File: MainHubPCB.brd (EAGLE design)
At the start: 100 x 80.3 mm, 77 parts, among them Q1 600mA/40V, Q2 600mA/40V, Q3 600mA/40V, U1 HX711, U2 HX711, U4 STM32F0XXC1T, U5 PCF8574T/3,512SOT162-1-M, U6 HX711

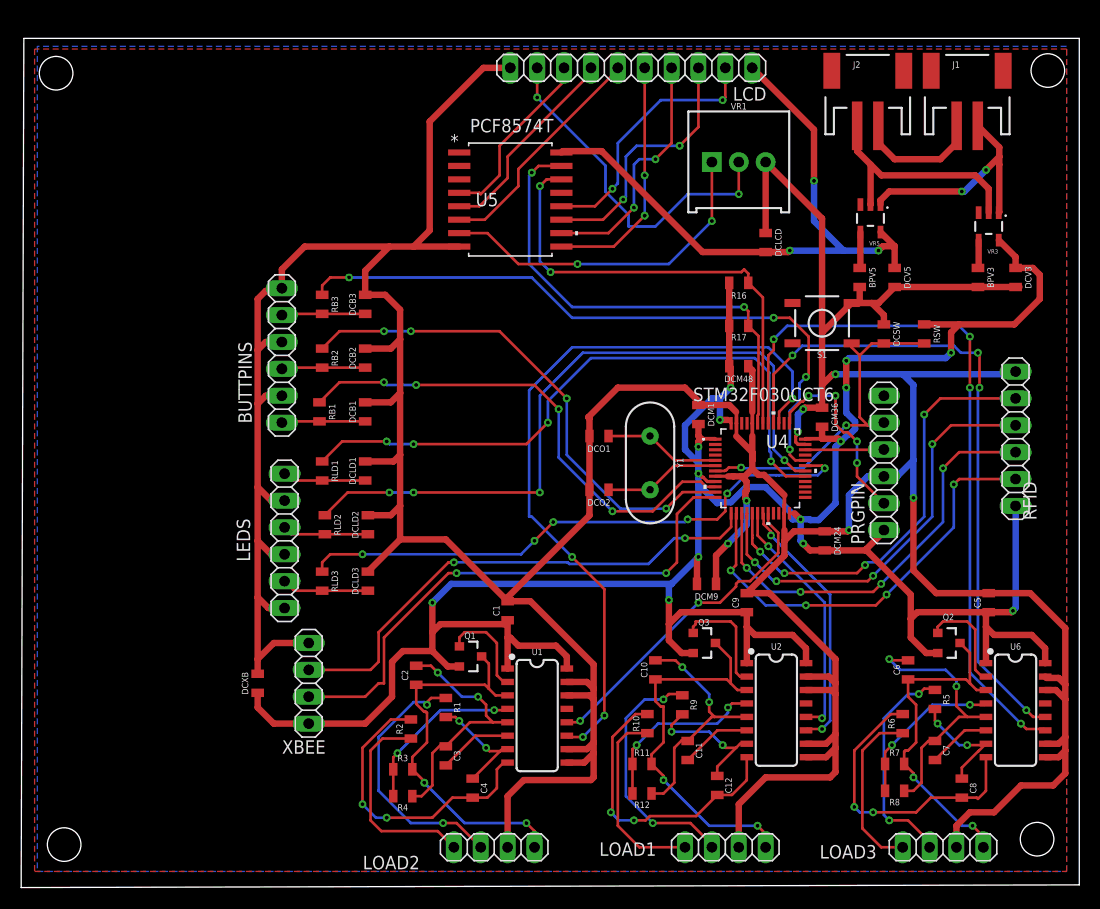
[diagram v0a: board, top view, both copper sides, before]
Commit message: final stuff
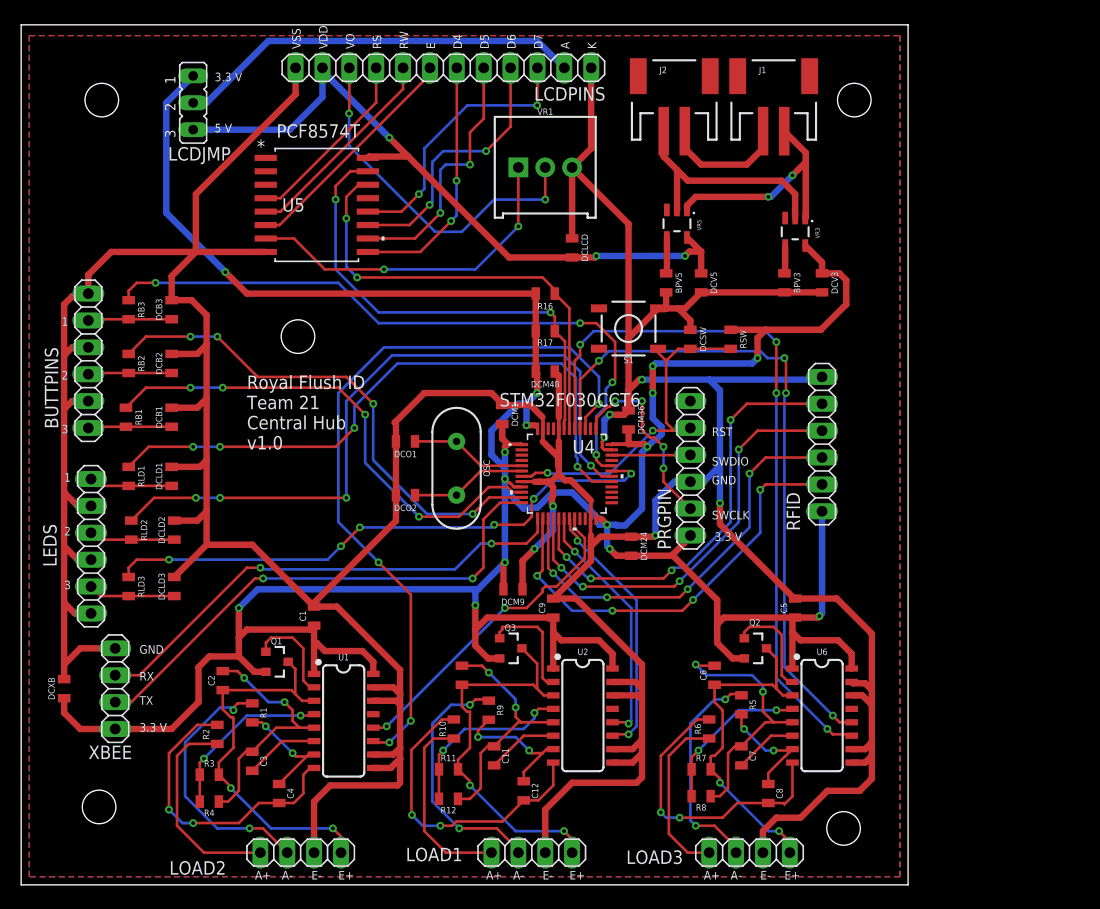
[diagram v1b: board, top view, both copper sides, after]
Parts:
- removed LCD: (no value), pinhead:1X10
- removed Y1: (no value), SparkFun-Clocks:HC49US
- added LCDJMP: (no value), jumper:JP2
- added LCDPINS: (no value), pinhead:1X12
- added OSC: (no value), SparkFun-Clocks:HC49US
- moved DCM1 18.5 mm to (45.5, 44.5)
- moved R16 18.3 mm to (49.5, 55.9)
- moved BPV3 18.3 mm to (72.1, 56.9)
- moved C8 18.3 mm to (70.6, 8.64)
- moved DCV3 18.3 mm to (75.7, 56.9)
- moved RFID 18.3 mm to (75.7, 41.7)
- moved U6 18.3 mm to (75.7, 16.0)
- moved BPV5 18.3 mm to (61.0, 56.9)
- moved BUTTPINS 18.3 mm to (6.35, 49.5)
- moved C10 18.3 mm to (41.7, 19.8)
- moved C12 18.3 mm to (47.5, 8.89)
- moved DCLCD 18.3 mm to (52.1, 60.2)
- moved DCSW 18.3 mm to (63.2, 51.6)
- moved J2 18.3 mm to (61.7, 74.9)
- moved LOAD1 18.3 mm to (48.3, 3.05)
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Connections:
- net A2 renamed TX
- net A3 renamed RX
- net B6 renamed SCL
- net B7 renamed SDA
- net N$12 renamed 3_A-
- net N$13 renamed 3_A+
- net N$17 renamed 3_VDD
- net N$2 renamed 2_A-
- net N$23 renamed 1_A-
- net N$24 renamed 1_A+
- net N$28 renamed 1_VDD
- net N$3 renamed 2_A+
- net N$7 renamed 2_VDD
- removed net B: LCD.9, VR1.2
- removed net D0: LCD.8, U5.4
- removed net D1: LCD.7, U5.5
- removed net D2: LCD.6, U5.6
- new net E: LCDPINS.7, U5.6
- new net POT_A: U5.7, VR1.1
- new net POT_B: LCDPINS.10, VR1.2
- new net RS: LCDPINS.9, U5.4
- new net RW: LCDPINS.8, U5.5
- net A: now also LCDJMP.2, LCDPINS.2; no longer U5.7, VR1.1
- net D4: now also LCDPINS.6; no longer LCD.5
- net D5: now also LCDPINS.5; no longer LCD.4
- net D6: now also LCDPINS.4; no longer LCD.3
- net D7: now also LCDPINS.3; no longer LCD.2
- net GND: now also LCDPINS.1, LCDPINS.12; no longer LCD.10
- net N$21: now also OSC.1; no longer Y1.1
- net N$22: now also OSC.2; no longer Y1.2
- net P3V: now also LCDJMP.1
- net P5V: now also LCDJMP.3, LCDPINS.11; no longer LCD.1
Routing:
- net P3V: track 275.7 -> 328.2 mm, vias 14 -> 15
- net POT_B: track 0.00 -> 33.6 mm, vias 0 -> 2
- net B: track 33.3 -> 0.00 mm, vias 2 -> 0
- net POT_A: track 0.00 -> 32.3 mm, vias 0 -> 2
- net E: track 0.00 -> 22.1 mm
- net D2: track 22.0 -> 0.00 mm
- net RW: track 0.00 -> 19.8 mm
- net D1: track 19.4 -> 0.00 mm
- net RS: track 0.00 -> 17.5 mm
- net D0: track 17.3 -> 0.00 mm
- net P5V: track 60.5 -> 67.7 mm
- net A: track 32.3 -> 38.5 mm, vias 2 -> 0
- net GND: track 510.6 -> 515.8 mm
- net TX: track 51.4 -> 48.9 mm
- net RX: track 48.6 -> 46.9 mm
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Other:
- board size 100 x 80.3 mm -> 83.8 x 81.3 mm
- board text added: "1"
- board text added: "2"
- board text added: "3"
- board text added: "3.3 V"
- board text added: "5 V"
- board text added: "A"
- board text added: "A+"
- board text added: "A-"
- board text added: "D4"
- board text added: "D5"
- board text added: "D6"
- board text added: "D7"
- board text added: "E"
- board text added: "E+"
- board text added: "E-"
- board text added: "GND"
- board text added: "K"
- board text added: "RS"
- board text added: "RST"
- board text added: "RW"
- board text added: "RX"
- board text added: "Royal Flush ID Team 21 Central Hub v1.0"
- board text added: "SWCLK"
- board text added: "SWDIO"
- board text added: "TX"
- board text added: "VDD"
- board text added: "VO"
- board text added: "VSS"
